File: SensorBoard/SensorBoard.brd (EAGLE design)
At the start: 136.2 x 101 mm, 74 parts, among them IC1 7805, J1 DCJ0202, X1 gen1, X13 3.3out1, X14 3.3out2, X15 uart1, X16 uart2, X17 uart3, X18 uart4, X2 motordriver1, X4 gen2, X5 gen3, X6 gen4, X7 programmer, X8 motordriver2

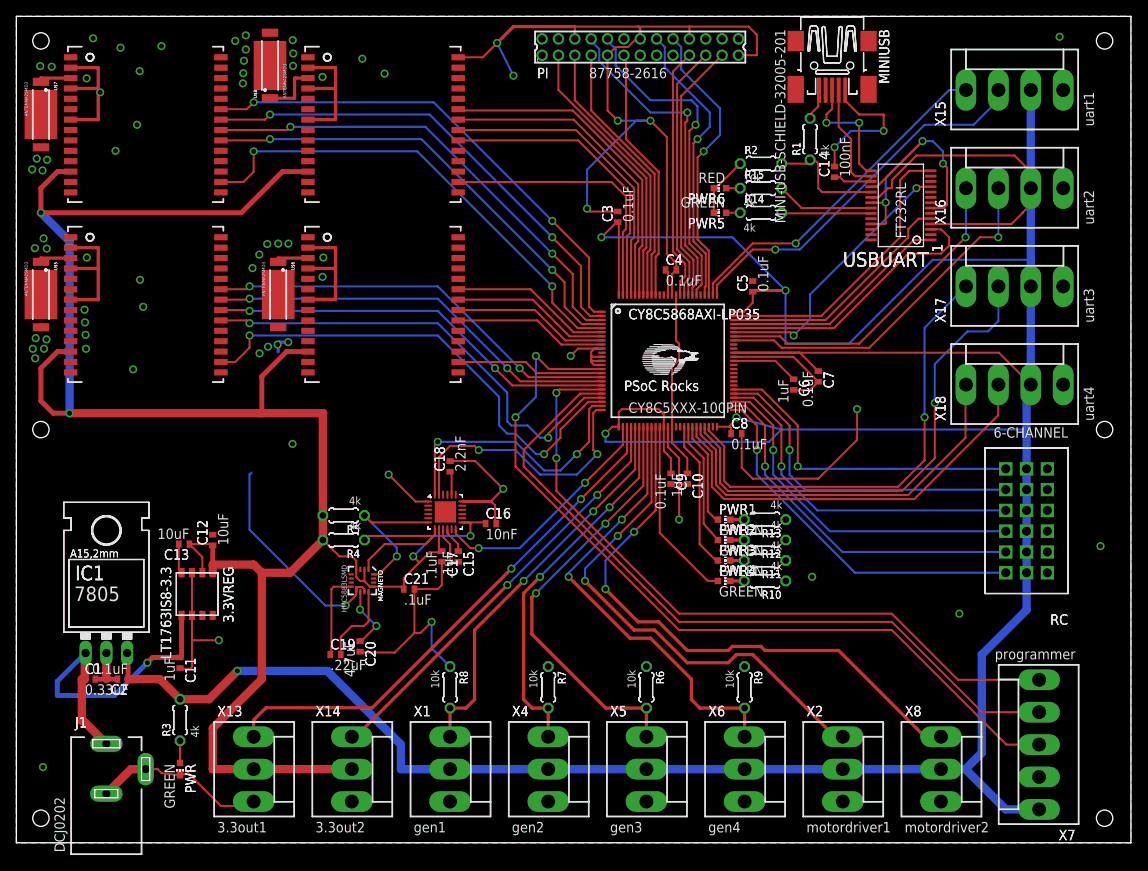
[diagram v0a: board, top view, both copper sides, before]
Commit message: okay now im done.
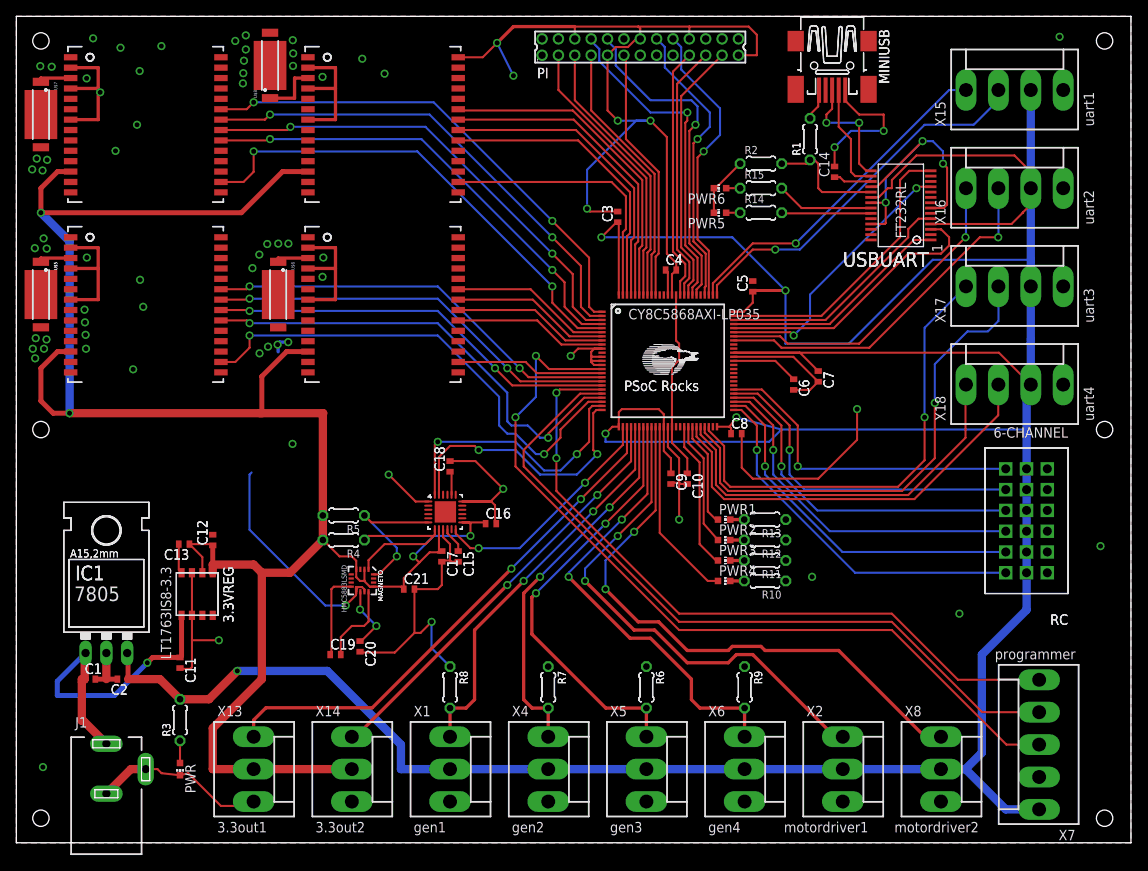
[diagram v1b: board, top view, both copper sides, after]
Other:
- board text removed: ".1uF"
- board text removed: ".22uF"
- board text removed: "0.1uF"
- board text removed: "0.33uF"
- board text removed: "100nF"
- board text removed: "10k"
- board text removed: "10nF"
- board text removed: "10uF"
- board text removed: "1uF"
- board text removed: "2.2nF"
- board text removed: "4.7uF"
- board text removed: "4k"
- board text removed: "87758-2616"
- board text removed: "ANTENNA2SMD3"
- board text removed: "C14"
- board text removed: "CY8C5868AXI-LP035"
- board text removed: "CY8C5XXX-100PIN"
- board text removed: "DCJ0202"
- board text removed: "GREEN"
- board text removed: "J1"
- board text removed: "LT1763IS8-3.3"
- board text removed: "MINI-USB-SCHIELD-32005-201"
- board text removed: "PWR"
- board text removed: "PWR1"
- board text removed: "PWR2"
- board text removed: "PWR3"
- board text removed: "PWR4"
- board text removed: "PWR5"
- board text removed: "PWR6"
- board text removed: "R10"
- board text removed: "R11"
- board text removed: "R12"
- board text removed: "R13"
- board text removed: "R14"
- board text removed: "R15"
- board text removed: "R2"
- board text removed: "R4"
- board text removed: "R5"
- board text removed: "RED"
- board text removed: "U$6"
- board text removed: "U$7"
- board text removed: "U$8"
- board text removed: "X1"
- board text removed: "X13"
- board text removed: "X14"
- board text removed: "X15"
- board text removed: "X16"
- board text removed: "X17"
- board text removed: "X18"
- board text removed: "X2"
- board text removed: "X4"
- board text removed: "X5"
- board text removed: "X6"
- board text removed: "X7"
- board text removed: "X8"
